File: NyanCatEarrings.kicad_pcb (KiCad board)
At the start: 2 copper layers, 26.6 x 17.9 mm, 12 parts, among them IC1 ATTINY10-TS, P1 G, P2 V, P4 I, P5 C, P6 R

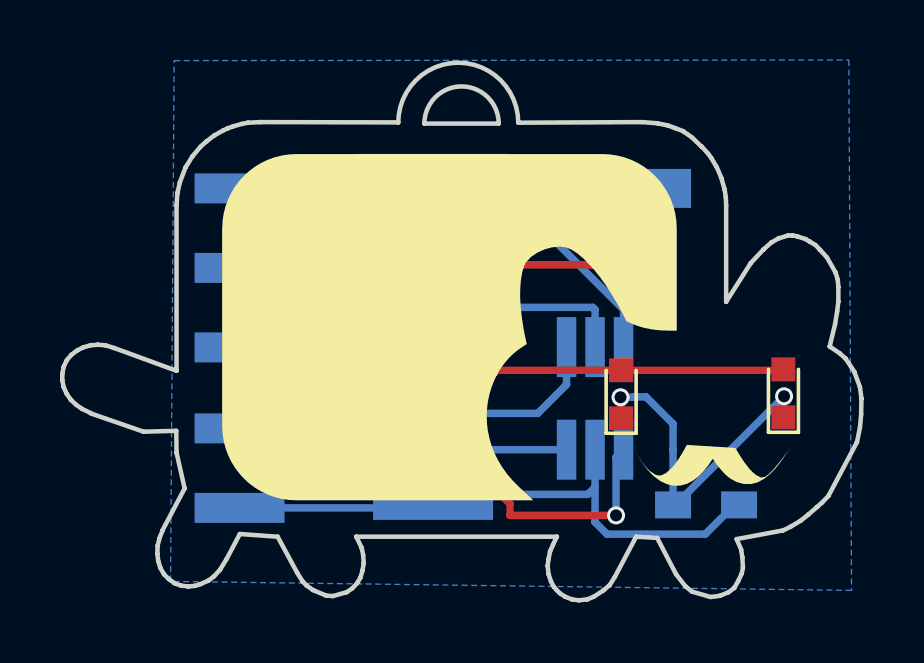
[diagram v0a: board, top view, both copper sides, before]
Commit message: Optimized tracks
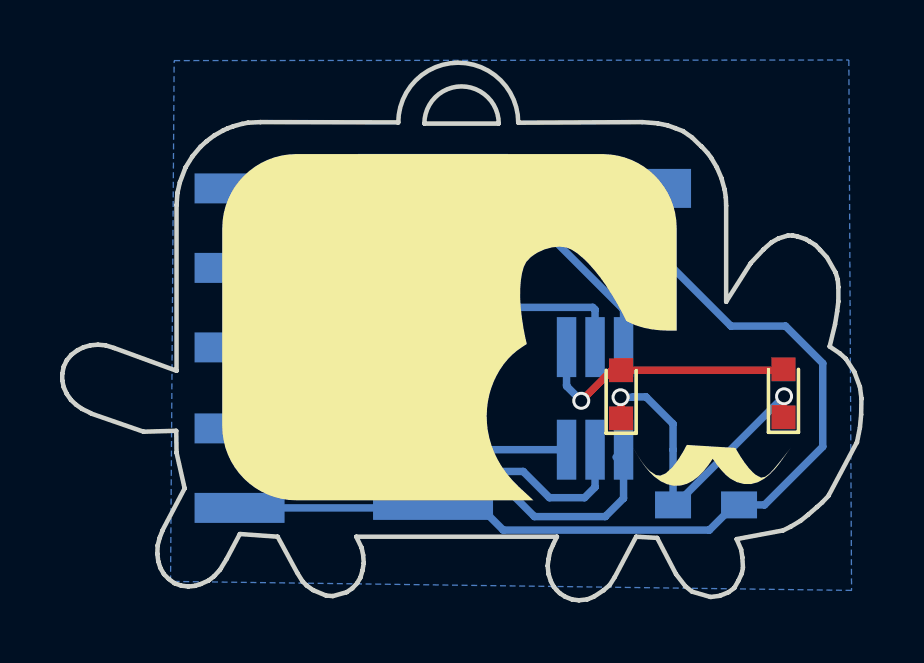
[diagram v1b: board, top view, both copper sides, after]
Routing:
- net GND: track 19.9 -> 40.6 mm
- net Net-(D1-Pad2): track 17.0 -> 9.22 mm
- net Net-(BZ1-Pad1): track 28.3 -> 27.2 mm
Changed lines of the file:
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@@
   (general
     (links 14)
-    (no_connects 0)
+    (no_connects 4)
     (area 128.614999 65.834999 155.405001 83.905001)
     (thickness 1.6)
     (drawings 160)
-    (tracks 87)
+    (tracks 100)
     (zones 0)
     (modules 12)
@@
   )
   (page A4)
+  (title_block
+    (title NyanCatEarrings)
+    (date 2018-03-10)
+    (rev 0.2)
+    (company "Electronic Cats")
+    (comment 1 "Andres Sabas")
+  )
   (layers
     (0 F.Cu signal)
@@
     (37 F.SilkS user)
     (38 B.Mask user)
-    (39 F.Mask user)
+    (39 F.Mask user hide)
     (40 Dwgs.User user)
     (41 Cmts.User user)
@@
     (46 B.CrtYd user)
     (47 F.CrtYd user)
-    (48 B.Fab user)
+    (48 B.Fab user hide)
     (49 F.Fab user)
   )
@@
   (gr_line (start 154.24 80.33) (end 155.18 78.56) (layer Edge.Cuts) (width 0.15))
   (gr_line (start 151.17 81.79) (end 152.72 81.5) (layer Edge.Cuts) (width 0.15))
+  (segment (start 144.48 70.09) (end 146.19 70.09) (width 0.25) (layer B.Cu) (net 1))
+  (segment (start 146.19 70.09) (end 146.2 70.1) (width 0.25) (layer B.Cu) (net 1))
+  (segment (start 143.42 72.65) (end 144.48 71.59) (width 0.25) (layer F.Cu) (net 1))
+  (segment (start 144.48 71.59) (end 144.48 70.09) (width 0.25) (layer F.Cu) (net 1))
+  (via (at 144.48 70.09) (size 0.6) (drill 0.4) (layers F.Cu B.Cu) (net 1))
+  (segment (start 142.45 72.65) (end 143.42 72.65) (width 0.25) (layer F.Cu) (net 1))
   (segment (start 142.45 72.65) (end 137.35 72.65) (width 0.25) (layer B.Cu) (net 1))
   (segment (start 137.35 72.65) (end 136.35 73.65) (width 0.25) (layer B.Cu) (net 1))
@@
   (segment (start 136.35 74.65) (end 135.6 75.4) (width 0.25) (layer B.Cu) (net 1))
   (segment (start 135.6 75.4) (end 134.6 75.4) (width 0.25) (layer B.Cu) (net 1))
-  (segment (start 146.75 72.25) (end 146.35 72.65) (width 0.25) (layer F.Cu) (net 1))
-  (segment (start 146.35 72.65) (end 142.45 72.65) (width 0.25) (layer F.Cu) (net 1))
   (via (at 142.45 72.65) (size 0.6) (drill 0.4) (layers F.Cu B.Cu) (net 1))
-  (segment (start 146.2 70.1) (end 146.2 71.7) (width 0.25) (layer B.Cu) (net 1))
-  (segment (start 146.2 71.7) (end 146.75 72.25) (width 0.25) (layer B.Cu) (net 1))
-  (via (at 146.75 72.25) (size 0.6) (drill 0.4) (layers F.Cu B.Cu) (net 1))
   (segment (start 145.5 78.81) (end 138.01 78.81) (width 0.25) (layer B.Cu) (net 1))
   (segment (start 138.01 78.81) (end 136.35 77.15) (width 0.25) (layer B.Cu) (net 1))
   (segment (start 136.35 77.15) (end 136.35 76.15) (width 0.25) (layer B.Cu) (net 1))
   (segment (start 136.35 76.15) (end 135.6 75.4) (width 0.25) (layer B.Cu) (net 1))
-  (segment (start 151.25 80.65) (end 151.1 80.65) (width 0.25) (layer B.Cu) (net 2))
-  (segment (start 150.124999 81.625001) (end 146.849999 81.625001) (width 0.25) (layer B.Cu) (net 2))
-  (segment (start 151.1 80.65) (end 150.124999 81.625001) (width 0.25) (layer B.Cu) (net 2))
-  (segment (start 146.849999 81.625001) (end 146.45 81.225002) (width 0.25) (layer B.Cu) (net 2))
+  (segment (start 150.98 74.69) (end 148.9 72.61) (width 0.25) (layer B.Cu) (net 2))
+  (segment (start 148.9 72.61) (end 148.9 70.1) (width 0.25) (layer B.Cu) (net 2))
+  (segment (start 152.8 74.69) (end 150.98 74.69) (width 0.25) (layer B.Cu) (net 2))
+  (segment (start 154.04 75.93) (end 152.8 74.69) (width 0.25) (layer B.Cu) (net 2))
+  (segment (start 154.04 78.71) (end 154.04 75.93) (width 0.25) (layer B.Cu) (net 2))
+  (segment (start 151.25 80.65) (end 152.1 80.65) (width 0.25) (layer B.Cu) (net 2))
+  (segment (start 152.1 80.65) (end 154.04 78.71) (width 0.25) (layer B.Cu) (net 2))
+  (segment (start 144.93 80.41) (end 146.1 80.41) (width 0.25) (layer B.Cu) (net 2))
+  (segment (start 146.1 80.41) (end 146.45 80.06) (width 0.25) (layer B.Cu) (net 2))
   (segment (start 146.45 80.06) (end 146.45 78.81) (width 0.25) (layer B.Cu) (net 2))
-  (segment (start 146.45 81.225002) (end 146.45 80.06) (width 0.25) (layer B.Cu) (net 2))
+  (segment (start 144.054999 79.534999) (end 144.93 80.41) (width 0.25) (layer B.Cu) (net 2))
+  (segment (start 141.05 80.3) (end 142.484998 80.3) (width 0.25) (layer B.Cu) (net 2))
+  (segment (start 142.484998 80.3) (end 143.249999 79.534999) (width 0.25) (layer B.Cu) (net 2))
+  (segment (start 143.249999 79.534999) (end 144.054999 79.534999) (width 0.25) (layer B.Cu) (net 2))
+  (segment (start 141.05 80.3) (end 142.2 80.3) (width 0.25) (layer B.Cu) (net 2))
+  (segment (start 142.2 80.3) (end 143.39001 81.49001) (width 0.25) (layer B.Cu) (net 2))
+  (segment (start 143.39001 81.49001) (end 150.25999 81.49001) (width 0.25) (layer B.Cu) (net 2))
+  (segment (start 150.25999 81.49001) (end 151.1 80.65) (width 0.25) (layer B.Cu) (net 2))
+  (segment (start 151.1 80.65) (end 151.25 80.65) (width 0.25) (layer B.Cu) (net 2))
   (segment (start 134.6 80.75) (end 140.6 80.75) (width 0.25) (layer B.Cu) (net 2))
   (segment (start 140.6 80.75) (end 141.05 80.3) (width 0.25) (layer B.Cu) (net 2))
-  (segment (start 146.45 80.06) (end 146.21 80.3) (width 0.25) (layer B.Cu) (net 2))
-  (segment (start 146.21 80.3) (end 143.3 80.3) (width 0.25) (layer B.Cu) (net 2))
-  (segment (start 143.3 80.3) (end 141.05 80.3) (width 0.25) (layer B.Cu) (net 2))
-  (segment (start 141.75 77.6) (end 143.188 76.162) (width 0.25) (layer F.Cu) (net 3))
-  (segment (start 143.188 76.162) (end 147.32 76.162) (width 0.25) (layer F.Cu) (net 3))
+  (segment (start 145.99 77.18) (end 147.008 76.162) (width 0.25) (layer F.Cu) (net 3))
+  (segment (start 147.008 76.162) (end 147.32 76.162) (width 0.25) (layer F.Cu) (net 3))
+  (segment (start 145.5 76.64) (end 145.5 76.69) (width 0.25) (layer B.Cu) (net 3))
+  (segment (start 145.5 76.69) (end 145.99 77.18) (width 0.25) (layer B.Cu) (net 3))
+  (via (at 145.99 77.18) (size 0.6) (drill 0.4) (layers F.Cu B.Cu) (net 3))
+  (segment (start 147.32 76.162) (end 152.698 76.162) (width 0.25) (layer F.Cu) (net 3))
   (segment (start 145.5 75.39) (end 145.5 76.64) (width 0.25) (layer B.Cu) (net 3))
-  (segment (start 145.5 76.64) (end 144.54 77.6) (width 0.25) (layer B.Cu) (net 3))
-  (segment (start 144.54 77.6) (end 141.75 77.6) (width 0.25) (layer B.Cu) (net 3))
-  (via (at 141.75 77.6) (size 0.6) (drill 0.4) (layers F.Cu B.Cu) (net 3))
-  (segment (start 147.32 76.162) (end 152.698 76.162) (width 0.25) (layer F.Cu) (net 3))
   (segment (start 152.698 76.162) (end 152.73 76.13) (width 0.25) (layer F.Cu) (net 3))
   (segment (start 147.282 76.2) (end 147.32 76.162) (width 0.25) (layer F.Cu) (net 3))
@@
   (segment (start 137.525001 71.275001) (end 136.35 70.1) (width 0.25) (layer B.Cu) (net 6))
   (segment (start 136.35 70.1) (end 134.6 70.1) (width 0.25) (layer B.Cu) (net 6))
-  (segment (start 147.15 81) (end 147.15 79.06) (width 0.25) (layer B.Cu) (net 7))
+  (segment (start 143.55 80.16) (end 144.43 81.04) (width 0.25) (layer B.Cu) (net 7))
+  (segment (start 144.43 81.04) (end 146.79 81.04) (width 0.25) (layer B.Cu) (net 7))
+  (segment (start 146.79 81.04) (end 147.4 80.43) (width 0.25) (layer B.Cu) (net 7))
+  (segment (start 147.4 80.43) (end 147.4 78.81) (width 0.25) (layer B.Cu) (net 7))
+  (segment (start 141.05 78.05) (end 143.16 80.16) (width 0.25) (layer F.Cu) (net 7))
+  (segment (start 143.16 80.16) (end 143.55 80.16) (width 0.25) (layer F.Cu) (net 7))
+  (via (at 143.55 80.16) (size 0.6) (drill 0.4) (layers F.Cu B.Cu) (net 7))
   (segment (start 147.15 79.06) (end 147.4 78.81) (width 0.25) (layer B.Cu) (net 7))
-  (segment (start 141.05 78.05) (end 143.615 80.615) (width 0.25) (layer F.Cu) (net 7))
-  (segment (start 143.615 80.615) (end 143.615 81) (width 0.25) (layer F.Cu) (net 7))
   (segment (start 139.965 77.35) (end 140.35 77.35) (width 0.25) (layer B.Cu) (net 7))
   (segment (start 140.35 77.35) (end 141.05 78.05) (width 0.25) (layer B.Cu) (net 7))
   (via (at 141.05 78.05) (size 0.6) (drill 0.4) (layers F.Cu B.Cu) (net 7))
-  (segment (start 143.615 81) (end 147.15 81) (width 0.25) (layer F.Cu) (net 7))
-  (via (at 147.15 81) (size 0.6) (drill 0.4) (layers F.Cu B.Cu) (net 7))
   (segment (start 139.2 77.35) (end 139.965 77.35) (width 0.25) (layer B.Cu) (net 7))
   (segment (start 137 71.95) (end 137 75.15) (width 0.25) (layer F.Cu) (net 7))
